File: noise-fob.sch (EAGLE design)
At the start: 10 parts

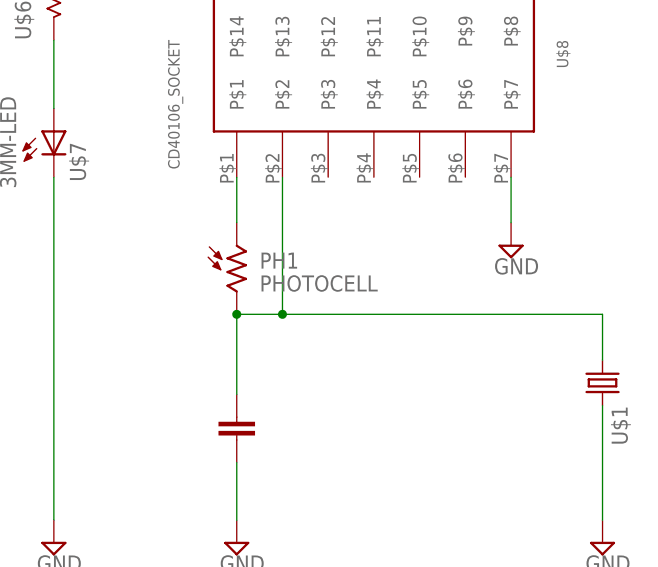
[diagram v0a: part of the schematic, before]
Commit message: updates
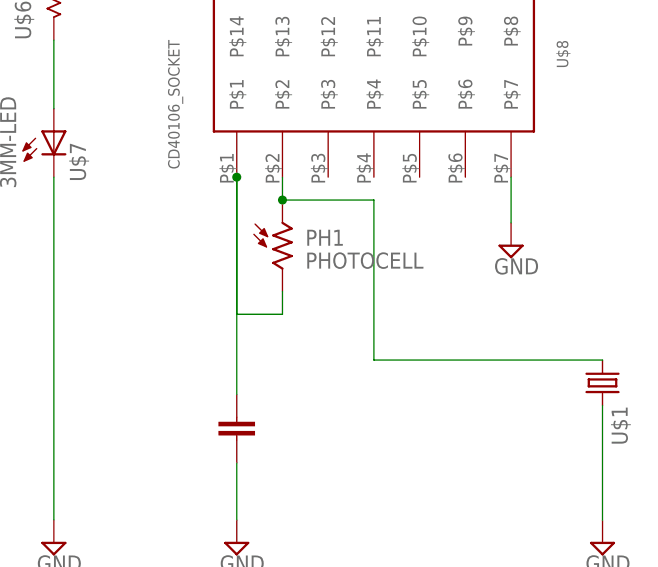
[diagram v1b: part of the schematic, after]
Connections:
- net N$5: now also U$1.1, U$8.P$2; no longer U$8.P$1
- net N$6: now also U$8.P$1; no longer U$1.1, U$8.P$2
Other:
- moved on the sheet: PH1
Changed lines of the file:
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@@
 <setting verticaltext="up"/>
 </settings>
-<grid distance="0.1" unitdist="inch" unit="inch" style="lines" multiple="1" display="yes" altdistance="0.01" altunitdist="inch" altunit="inch"/>
+<grid distance="0.1" unitdist="inch" unit="inch" style="lines" multiple="1" display="no" altdistance="0.01" altunitdist="inch" altunit="inch"/>
 <layers>
 <layer number="1" name="Top" color="4" fill="1" visible="no" active="no"/>
@@
 <attribute name="VALUE" x="130.175" y="4.445" size="1.778" layer="96"/>
 </instance>
-<instance part="PH1" gate="G$1" x="101.6" y="5.08" smashed="yes">
-<attribute name="NAME" x="104.14" y="5.08" size="1.778" layer="95"/>
-<attribute name="VALUE" x="104.14" y="2.54" size="1.778" layer="96"/>
+<instance part="PH1" gate="G$1" x="106.68" y="7.62" smashed="yes">
+<attribute name="NAME" x="109.22" y="7.62" size="1.778" layer="95"/>
+<attribute name="VALUE" x="109.22" y="5.08" size="1.778" layer="96"/>
 </instance>
 </instances>
@@
 </segment>
 </net>
-<net name="N$5" class="0">
-<segment>
-<pinref part="U$8" gate="G$1" pin="P$1"/>
-<wire x1="101.6" y1="10.16" x2="101.6" y2="15.24" width="0.1524" layer="91"/>
-<pinref part="PH1" gate="G$1" pin="1"/>
-</segment>
-</net>
-<net name="N$6" class="0">
-<segment>
-<wire x1="101.6" y1="0" x2="106.68" y2="0" width="0.1524" layer="91"/>
-<pinref part="U$8" gate="G$1" pin="P$2"/>
-<wire x1="106.68" y1="0" x2="106.68" y2="15.24" width="0.1524" layer="91"/>
-<pinref part="U$10" gate="G$1" pin="2"/>
-<wire x1="101.6" y1="0" x2="101.6" y2="-8.89" width="0.1524" layer="91"/>
-<wire x1="106.68" y1="0" x2="142.24" y2="0" width="0.1524" layer="91"/>
-<junction x="106.68" y="0"/>
-<pinref part="U$1" gate="G$1" pin="1"/>
-<wire x1="142.24" y1="0" x2="142.24" y2="-5.08" width="0.1524" layer="91"/>
-<pinref part="PH1" gate="G$1" pin="2"/>
-<junction x="101.6" y="0"/>
-</segment>
-</net>
 <net name="GND" class="0">
 <segment>
@@
 </segment>
 </net>
+<net name="N$5" class="0">
+<segment>
+<pinref part="U$8" gate="G$1" pin="P$2"/>
+<pinref part="PH1" gate="G$1" pin="1"/>
+<wire x1="106.68" y1="15.24" x2="106.68" y2="12.7" width="0.1524" layer="91"/>
+<wire x1="106.68" y1="12.7" x2="116.84" y2="12.7" width="0.1524" layer="91"/>
+<wire x1="116.84" y1="12.7" x2="116.84" y2="-5.08" width="0.1524" layer="91"/>
+<junction x="106.68" y="12.7"/>
+<pinref part="U$1" gate="G$1" pin="1"/>
+<wire x1="116.84" y1="-5.08" x2="142.24" y2="-5.08" width="0.1524" layer="91"/>
+</segment>
+</net>
+<net name="N$6" class="0">
+<segment>
+<pinref part="PH1" gate="G$1" pin="2"/>
+<wire x1="106.68" y1="2.54" x2="106.68" y2="0" width="0.1524" layer="91"/>
+<pinref part="U$8" gate="G$1" pin="P$1"/>
+<wire x1="106.68" y1="0" x2="101.6" y2="0" width="0.1524" layer="91"/>
+<wire x1="101.6" y1="0" x2="101.6" y2="15.24" width="0.1524" layer="91"/>
+<pinref part="U$10" gate="G$1" pin="2"/>
+<wire x1="101.6" y1="15.24" x2="101.6" y2="-8.89" width="0.1524" layer="91"/>
+<junction x="101.6" y="15.24"/>
+</segment>
+</net>
